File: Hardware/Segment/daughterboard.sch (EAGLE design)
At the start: 62 parts, among them IC1 PBQ79656PAPTQ1, X1 5566-12, X2 5566-12, X3 5566-16

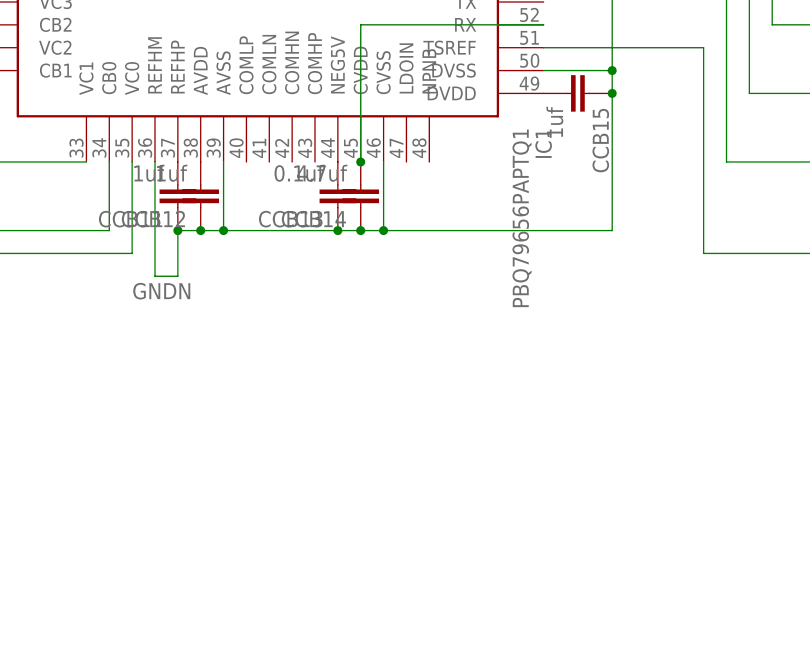
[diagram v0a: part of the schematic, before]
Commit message: Part of com
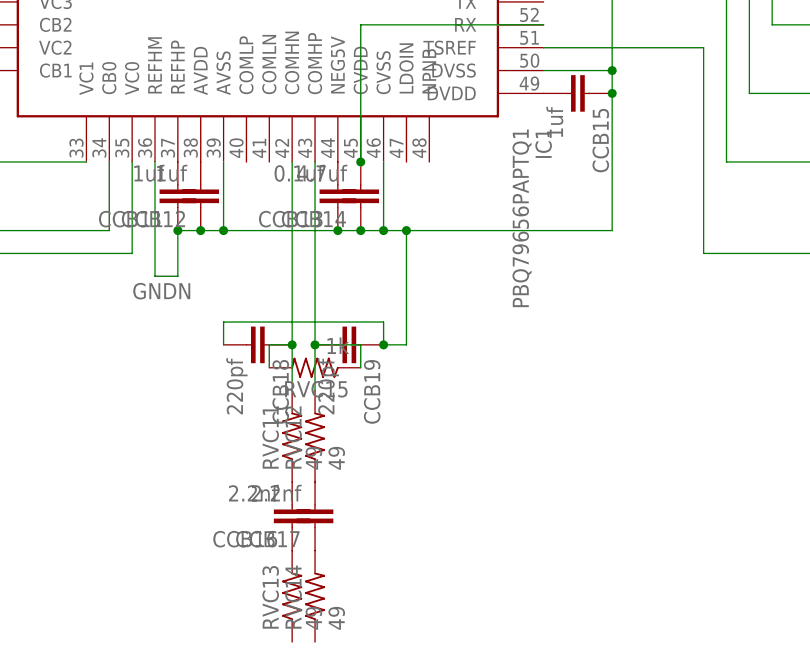
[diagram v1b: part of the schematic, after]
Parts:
- added CCB16, CCB17: 2.2nf, capacitor-wima:C2.5/2
- added CCB18, CCB19: 220pf, capacitor-wima:C2.5/2
- added RVC11, RVC12, RVC13, RVC14: 49, rcl:R-US_R0603
- added RVC15: 1k, rcl:R-US_R0603
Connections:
- new net N$59: CCB18.1, IC1.COMHN, RVC11.2, RVC15.2
- new net N$60: CCB19.2, IC1.COMHP, RVC12.2, RVC15.1
- new net N$61: CCB16.2, RVC11.1
- new net N$62: CCB17.2, RVC12.1
- new net N$63: CCB16.1, RVC13.2
- new net N$64: CCB17.1, RVC14.2
- net GNDN: now also CCB18.2, CCB19.1
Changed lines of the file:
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@@
 <part name="R7" library="rcl" library_urn="urn:adsk.eagle:library:334" deviceset="R-US_" device="R0603" package3d_urn="urn:adsk.eagle:package:23555/3" value="10k"/>
 <part name="R8" library="rcl" library_urn="urn:adsk.eagle:library:334" deviceset="R-US_" device="R0603" package3d_urn="urn:adsk.eagle:package:23555/3" value="10k"/>
+<part name="RVC11" library="rcl" library_urn="urn:adsk.eagle:library:334" deviceset="R-US_" device="R0603" package3d_urn="urn:adsk.eagle:package:23555/3" value="49"/>
+<part name="RVC12" library="rcl" library_urn="urn:adsk.eagle:library:334" deviceset="R-US_" device="R0603" package3d_urn="urn:adsk.eagle:package:23555/3" value="49"/>
+<part name="CCB16" library="capacitor-wima" library_urn="urn:adsk.eagle:library:116" deviceset="C" device="2.5/2" package3d_urn="urn:adsk.eagle:package:5415/1" value="2.2nf"/>
+<part name="CCB17" library="capacitor-wima" library_urn="urn:adsk.eagle:library:116" deviceset="C" device="2.5/2" package3d_urn="urn:adsk.eagle:package:5415/1" value="2.2nf"/>
+<part name="RVC13" library="rcl" library_urn="urn:adsk.eagle:library:334" deviceset="R-US_" device="R0603" package3d_urn="urn:adsk.eagle:package:23555/3" value="49"/>
+<part name="RVC14" library="rcl" library_urn="urn:adsk.eagle:library:334" deviceset="R-US_" device="R0603" package3d_urn="urn:adsk.eagle:package:23555/3" value="49"/>
+<part name="RVC15" library="rcl" library_urn="urn:adsk.eagle:library:334" deviceset="R-US_" device="R0603" package3d_urn="urn:adsk.eagle:package:23555/3" value="1k"/>
+<part name="CCB18" library="capacitor-wima" library_urn="urn:adsk.eagle:library:116" deviceset="C" device="2.5/2" package3d_urn="urn:adsk.eagle:package:5415/1" value="220pf"/>
+<part name="CCB19" library="capacitor-wima" library_urn="urn:adsk.eagle:library:116" deviceset="C" device="2.5/2" package3d_urn="urn:adsk.eagle:package:5415/1" value="220pf"/>
 </parts>
 <sheets>
@@
 <attribute name="NAME" x="240.03" y="77.6986" size="1.778" layer="95"/>
 <attribute name="VALUE" x="240.03" y="72.898" size="1.778" layer="96"/>
+</instance>
+<instance part="RVC11" gate="G$1" x="162.56" y="-2.54" smashed="yes" rot="R90">
+<attribute name="NAME" x="161.0614" y="-6.35" size="1.778" layer="95" rot="R90"/>
+<attribute name="VALUE" x="165.862" y="-6.35" size="1.778" layer="96" rot="R90"/>
+</instance>
+<instance part="RVC12" gate="G$1" x="165.1" y="-2.54" smashed="yes" rot="R90">
+<attribute name="NAME" x="163.6014" y="-6.35" size="1.778" layer="95" rot="R90"/>
+<attribute name="VALUE" x="168.402" y="-6.35" size="1.778" layer="96" rot="R90"/>
+</instance>
+<instance part="CCB16" gate="G$1" x="162.56" y="-12.7" smashed="yes" rot="R180">
+<attribute name="NAME" x="161.036" y="-13.081" size="1.778" layer="95" rot="R180"/>
+<attribute name="VALUE" x="161.036" y="-8.001" size="1.778" layer="96" rot="R180"/>
+</instance>
+<instance part="CCB17" gate="G$1" x="165.1" y="-12.7" smashed="yes" rot="R180">
+<attribute name="NAME" x="163.576" y="-13.081" size="1.778" layer="95" rot="R180"/>
+<attribute name="VALUE" x="163.576" y="-8.001" size="1.778" layer="96" rot="R180"/>
+</instance>
+<instance part="RVC13" gate="G$1" x="162.56" y="-20.32" smashed="yes" rot="R90">
+<attribute name="NAME" x="161.0614" y="-24.13" size="1.778" layer="95" rot="R90"/>
+<attribute name="VALUE" x="165.862" y="-24.13" size="1.778" layer="96" rot="R90"/>
+</instance>
+<instance part="RVC14" gate="G$1" x="165.1" y="-20.32" smashed="yes" rot="R90">
+<attribute name="NAME" x="163.6014" y="-24.13" size="1.778" layer="95" rot="R90"/>
+<attribute name="VALUE" x="168.402" y="-24.13" size="1.778" layer="96" rot="R90"/>
+</instance>
+<instance part="RVC15" gate="G$1" x="165.1" y="5.08" smashed="yes" rot="R180">
+<attribute name="NAME" x="168.91" y="3.5814" size="1.778" layer="95" rot="R180"/>
+<attribute name="VALUE" x="168.91" y="8.382" size="1.778" layer="96" rot="R180"/>
+</instance>
+<instance part="CCB18" gate="G$1" x="160.02" y="7.62" smashed="yes" rot="R270">
+<attribute name="NAME" x="160.401" y="6.096" size="1.778" layer="95" rot="R270"/>
+<attribute name="VALUE" x="155.321" y="6.096" size="1.778" layer="96" rot="R270"/>
+</instance>
+<instance part="CCB19" gate="G$1" x="170.18" y="7.62" smashed="yes" rot="R270">
+<attribute name="NAME" x="170.561" y="6.096" size="1.778" layer="95" rot="R270"/>
+<attribute name="VALUE" x="165.481" y="6.096" size="1.778" layer="96" rot="R270"/>
 </instance>
 </instances>
@@
 <wire x1="198.12" y1="38.1" x2="198.12" y2="35.56" width="0.1524" layer="91"/>
 <wire x1="198.12" y1="35.56" x2="198.12" y2="20.32" width="0.1524" layer="91"/>
-<wire x1="198.12" y1="20.32" x2="172.72" y2="20.32" width="0.1524" layer="91"/>
+<wire x1="198.12" y1="20.32" x2="175.26" y2="20.32" width="0.1524" layer="91"/>
 <junction x="198.12" y="35.56"/>
 <junction x="172.72" y="20.32"/>
 <pinref part="IC1" gate="G$1" pin="AVSS?"/>
+<wire x1="175.26" y1="20.32" x2="172.72" y2="20.32" width="0.1524" layer="91"/>
 <wire x1="190.5" y1="76.2" x2="198.12" y2="76.2" width="0.1524" layer="91"/>
 <wire x1="198.12" y1="76.2" x2="198.12" y2="38.1" width="0.1524" layer="91"/>
 <junction x="198.12" y="38.1"/>
+<pinref part="CCB18" gate="G$1" pin="2"/>
+<wire x1="154.94" y1="7.62" x2="154.94" y2="10.16" width="0.1524" layer="91"/>
+<pinref part="CCB19" gate="G$1" pin="1"/>
+<wire x1="154.94" y1="10.16" x2="172.72" y2="10.16" width="0.1524" layer="91"/>
+<wire x1="172.72" y1="10.16" x2="172.72" y2="7.62" width="0.1524" layer="91"/>
+<wire x1="172.72" y1="7.62" x2="175.26" y2="7.62" width="0.1524" layer="91"/>
+<wire x1="175.26" y1="7.62" x2="175.26" y2="20.32" width="0.1524" layer="91"/>
+<junction x="172.72" y="7.62"/>
+<junction x="175.26" y="20.32"/>
 </segment>
 </net>
@@
 </segment>
 </net>
+<net name="N$59" class="0">
+<segment>
+<pinref part="IC1" gate="G$1" pin="COMHN"/>
+<wire x1="162.56" y1="27.94" x2="162.56" y2="7.62" width="0.1524" layer="91"/>
+<pinref part="RVC11" gate="G$1" pin="2"/>
+<pinref part="RVC15" gate="G$1" pin="2"/>
+<wire x1="162.56" y1="7.62" x2="162.56" y2="2.54" width="0.1524" layer="91"/>
+<wire x1="160.02" y1="5.08" x2="160.02" y2="7.62" width="0.1524" layer="91"/>
+<wire x1="160.02" y1="7.62" x2="162.56" y2="7.62" width="0.1524" layer="91"/>
+<junction x="162.56" y="7.62"/>
+<pinref part="CCB18" gate="G$1" pin="1"/>
+</segment>
+</net>
+<net name="N$60" class="0">
+<segment>
+<pinref part="IC1" gate="G$1" pin="COMHP"/>
+<wire x1="165.1" y1="27.94" x2="165.1" y2="7.62" width="0.1524" layer="91"/>
+<pinref part="RVC12" gate="G$1" pin="2"/>
+<pinref part="RVC15" gate="G$1" pin="1"/>
+<wire x1="165.1" y1="7.62" x2="165.1" y2="2.54" width="0.1524" layer="91"/>
+<wire x1="170.18" y1="5.08" x2="170.18" y2="7.62" width="0.1524" layer="91"/>
+<wire x1="170.18" y1="7.62" x2="165.1" y2="7.62" width="0.1524" layer="91"/>
+<junction x="165.1" y="7.62"/>
+<pinref part="CCB19" gate="G$1" pin="2"/>
+</segment>
+</net>
+<net name="N$61" class="0">
+<segment>
+<pinref part="CCB16" gate="G$1" pin="2"/>
+<pinref part="RVC11" gate="G$1" pin="1"/>
+</segment>
+</net>
+<net name="N$62" class="0">
+<segment>
+<pinref part="CCB17" gate="G$1" pin="2"/>
+<pinref part="RVC12" gate="G$1" pin="1"/>
+</segment>
+</net>
+<net name="N$63" class="0">
+<segment>
+<pinref part="RVC13" gate="G$1" pin="2"/>
+<pinref part="CCB16" gate="G$1" pin="1"/>
+</segment>
+</net>
+<net name="N$64" class="0">
+<segment>
+<pinref part="RVC14" gate="G$1" pin="2"/>
+<pinref part="CCB17" gate="G$1" pin="1"/>
+</segment>
+</net>
